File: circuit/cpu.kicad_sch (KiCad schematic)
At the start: 27 parts, among them J1 Port B, J2 Port C, J3 Port E, J3 Port F, J4 Port A, J43 Port G, J5 Port D, U1 74HTC138, U6 74LS08

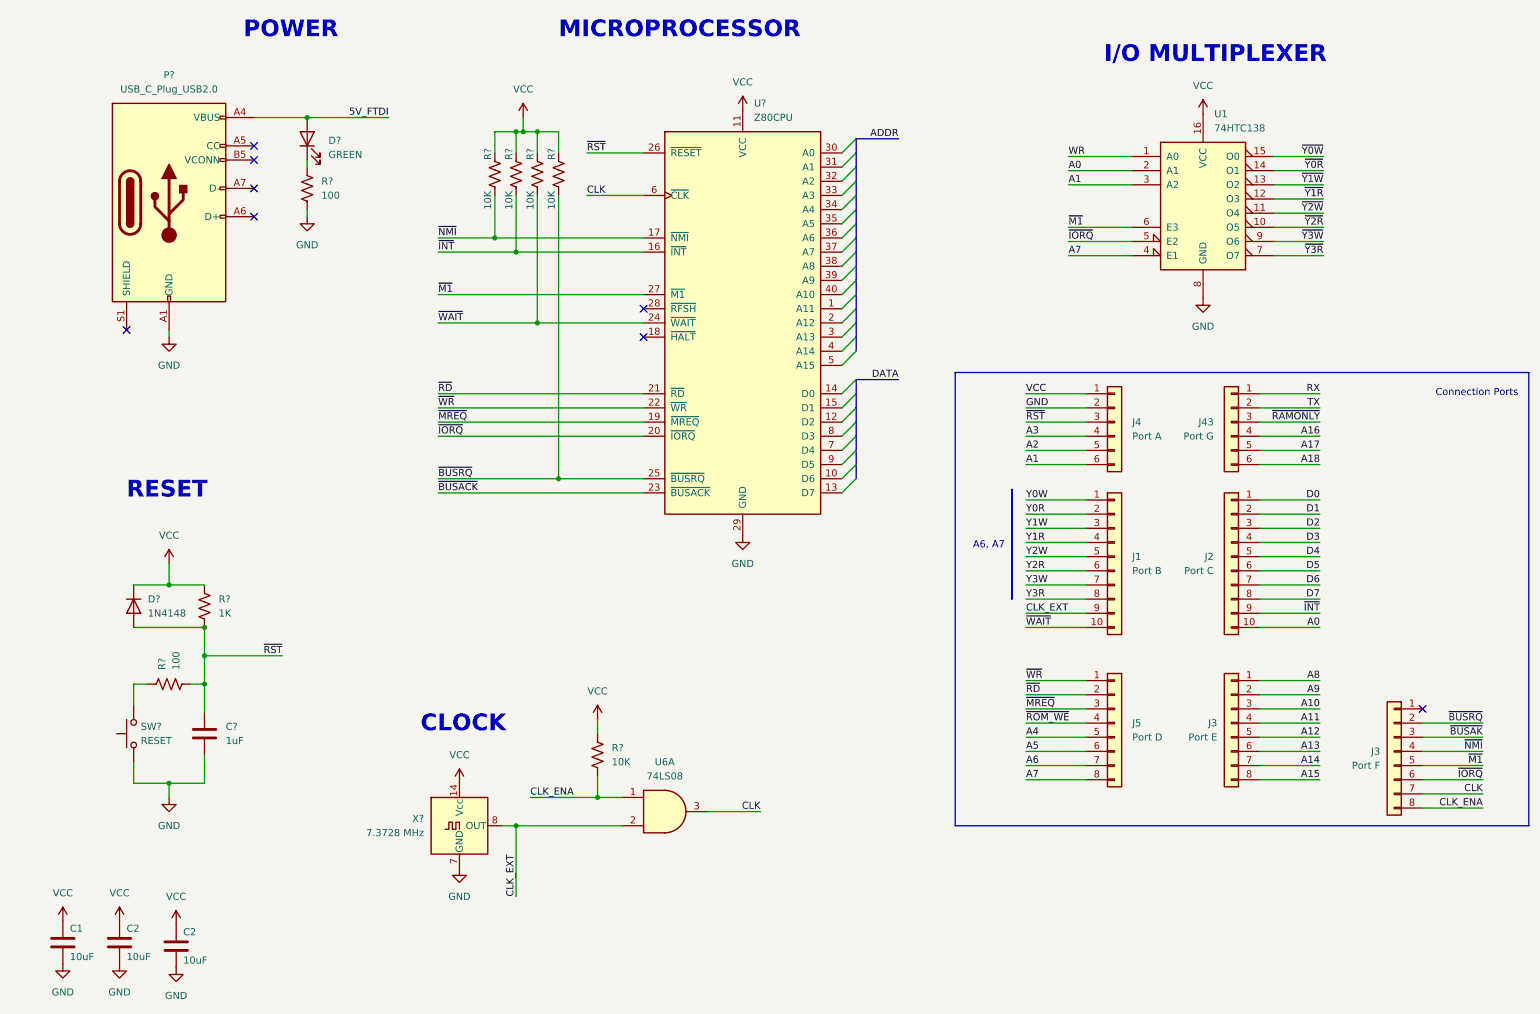
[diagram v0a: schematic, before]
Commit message: .
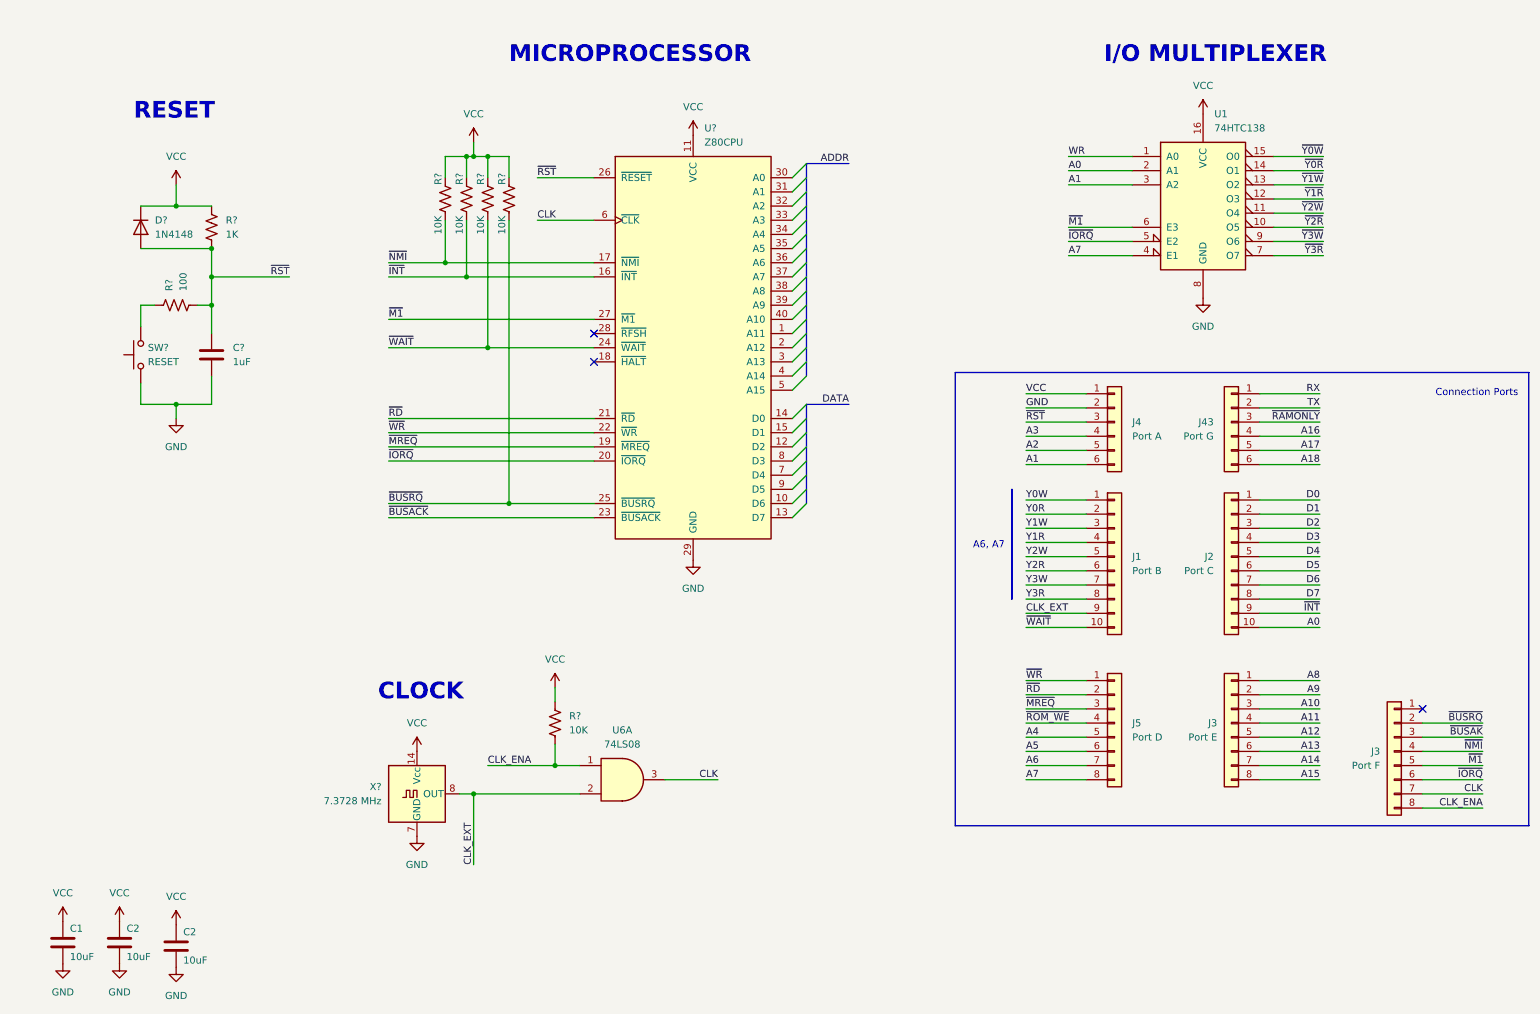
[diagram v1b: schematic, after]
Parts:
- removed D?: GREEN, symbol Device:LED
- removed P?: USB_C_Plug_USB2.0, symbol Connector:USB_C_Plug_USB2.0
- removed R?: 100, symbol Device:R_US
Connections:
- no-connect marks 8 -> 3
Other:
- note removed: "POWER"
- moved on the sheet: C?, D?, R?, SW?, U6A, U?, X?

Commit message: .
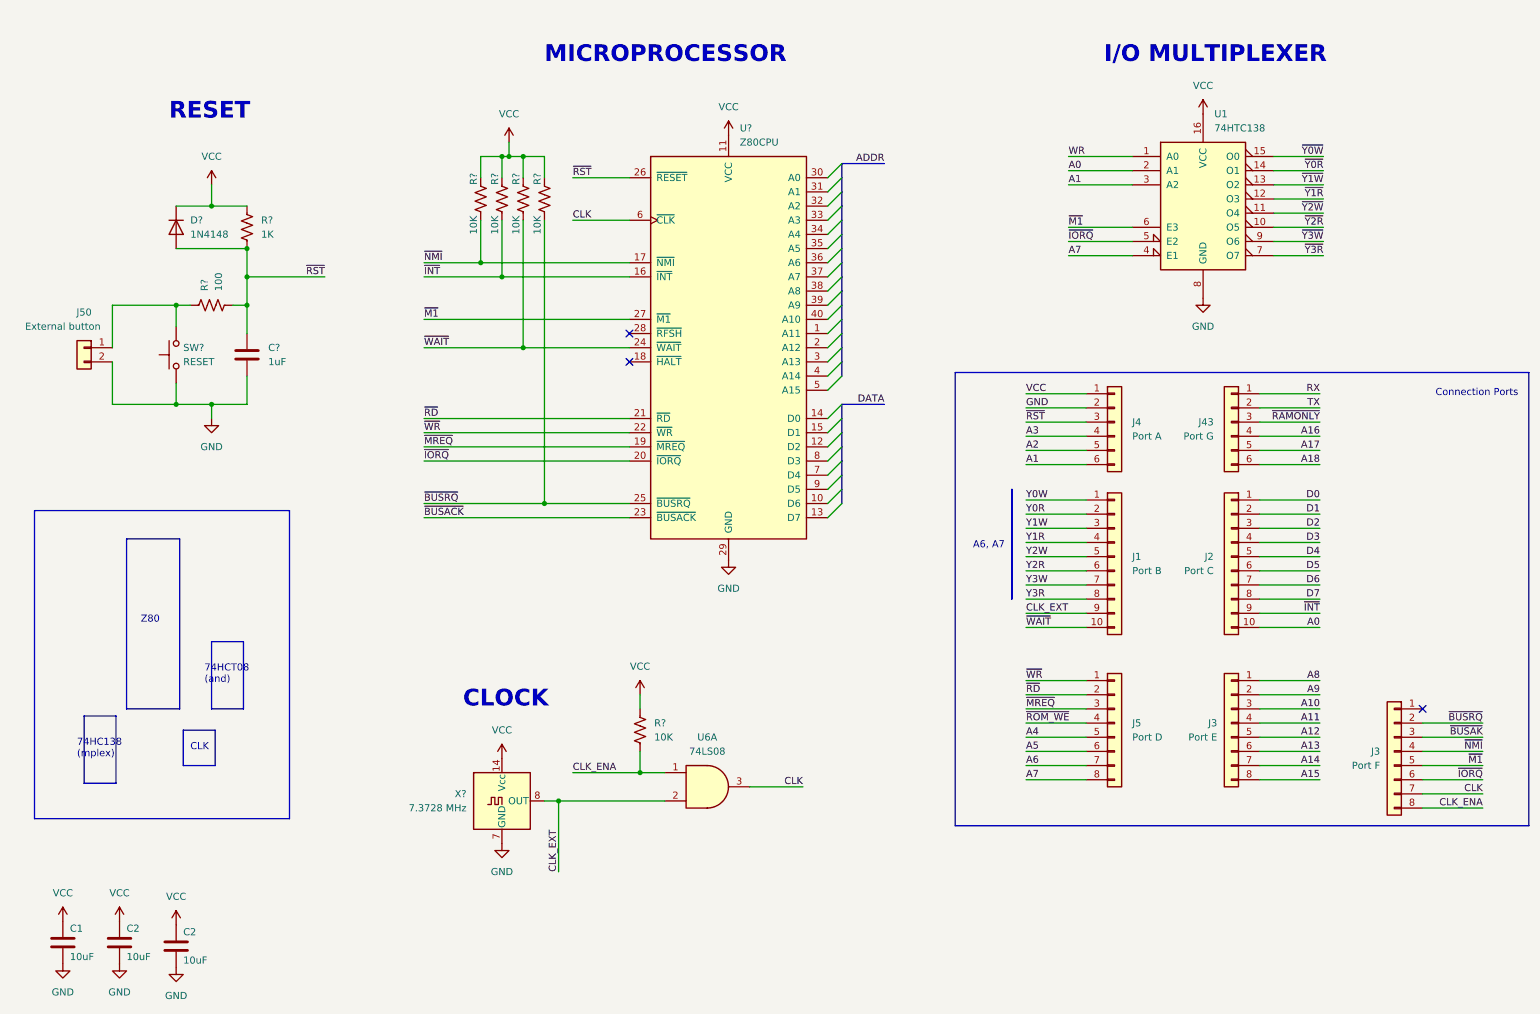
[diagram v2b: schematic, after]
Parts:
- added J50: External button, symbol Connector_Generic:Conn_01x02
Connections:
- net GND: now also J50.2 (Pin_2)
- net at R?.2, SW?.2: now also J50.1 (Pin_1)
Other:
- note added: "74HC138 (mplex)"
- note added: "74HCT08 (and)"
- note added: "CLK"
- note added: "Z80"
- moved on the sheet: C?, D?, R?, SW?, U6A, U?, X?
